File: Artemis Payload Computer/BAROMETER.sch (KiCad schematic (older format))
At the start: 1 part, among them U301 BMP280

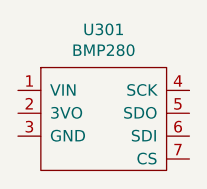
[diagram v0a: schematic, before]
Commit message: I think I undid this...
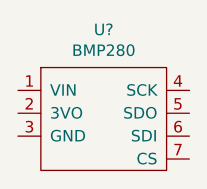
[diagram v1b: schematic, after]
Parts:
- renumbered U301 to U?
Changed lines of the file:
@@
 $Descr A4 11693 8268
 encoding utf-8
-Sheet 3 5
+Sheet 3 4
 Title ""
 Date ""
@@
 $EndDescr
 $Comp
-L Artemis_Footprints:BMP280 U301
+L Artemis_Footprints:BMP280 U?
 U 1 1 603A8ECA
 P 6100 3650
-F 0 "U301" H 6125 4015 50  0000 C CNN
+F 0 "U?" H 6125 4015 50  0000 C CNN
 F 1 "BMP280" H 6125 3924 50  0000 C CNN
 F 2 "" H 6100 4150 50  0001 C CNN

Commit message: Fuck it we're starting over. Sorry for the mess Nathan
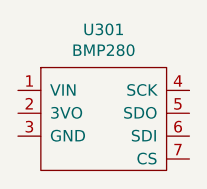
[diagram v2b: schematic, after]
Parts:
- gave numbers to parts that had none: 1
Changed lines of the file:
@@
 $Descr A4 11693 8268
 encoding utf-8
-Sheet 3 4
+Sheet 3 5
 Title ""
 Date ""
@@
 $EndDescr
 $Comp
-L Artemis_Footprints:BMP280 U?
+L Artemis_Footprints:BMP280 U301
 U 1 1 603A8ECA
 P 6100 3650
-F 0 "U?" H 6125 4015 50  0000 C CNN
+F 0 "U301" H 6125 4015 50  0000 C CNN
 F 1 "BMP280" H 6125 3924 50  0000 C CNN
 F 2 "" H 6100 4150 50  0001 C CNN
